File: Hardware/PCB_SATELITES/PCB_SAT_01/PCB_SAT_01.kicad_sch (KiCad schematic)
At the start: 41 parts, among them IC1 OPT3001DNPRQ1, IC2 OPT3001DNPRQ1, IC3 OPT3001DNPRQ1, IC4 OPT3001DNPRQ1, J1 MTJ-88ARX1-FSM-LG

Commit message: Actualizacion PCB SATELITE 1
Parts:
- C1, C2, C3, C4: footprint (none) -> Capacitor_SMD:C_0805_2012Metric
- J1: footprint MTJ88ARX1FSMLG -> MTJ-88ARX1-FSM-LG:MTJ88ARX1FSMLG
- R1, R10, R11, R12, R2, R3, R4, R5, R6, R7, R8, R9: footprint (none) -> Resistor_SMD:R_0805_2012Metric
- TP1_1, TP1_2, TP1_3, TP1_4, TP1_5, TP2_1, TP2_2, TP2_3, TP2_4, TP2_5, TP3_1, TP3_2, TP3_3, TP3_4, TP3_5, TP4_1, TP4_2, TP4_3, TP4_4, TP4_5: footprint (none) -> TestPoint:TestPoint_Pad_D1.0mm
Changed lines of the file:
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@@
 			)
 		)
-		(property "Footprint" ""
+		(property "Footprint" "TestPoint:TestPoint_Pad_D1.0mm"
 			(at 143.51 41.91 0)
 			(effects
@@
 			)
 		)
-		(property "Footprint" ""
+		(property "Footprint" "TestPoint:TestPoint_Pad_D1.0mm"
 			(at 92.71 49.53 0)
 			(effects
@@
 			)
 		)
-		(property "Footprint" ""
+		(property "Footprint" "TestPoint:TestPoint_Pad_D1.0mm"
 			(at 100.33 109.22 0)
 			(effects
@@
 			)
 		)
-		(property "Footprint" ""
+		(property "Footprint" "Capacitor_SMD:C_0805_2012Metric"
 			(at 155.9052 97.79 0)
 			(effects
@@
 			)
 		)
-		(property "Footprint" ""
+		(property "Footprint" "TestPoint:TestPoint_Pad_D1.0mm"
 			(at 186.69 52.07 0)
 			(effects
@@
 			)
 		)
-		(property "Footprint" ""
+		(property "Footprint" "TestPoint:TestPoint_Pad_D1.0mm"
 			(at 40.64 104.14 0)
 			(effects
@@
 			)
 		)
-		(property "Footprint" ""
+		(property "Footprint" "Capacitor_SMD:C_0805_2012Metric"
 			(at 50.4952 34.29 0)
 			(effects
@@
 			)
 		)
-		(property "Footprint" ""
+		(property "Footprint" "TestPoint:TestPoint_Pad_D1.0mm"
 			(at 195.58 49.53 0)
 			(effects
@@
 			)
 		)
-		(property "Footprint" ""
+		(property "Footprint" "Resistor_SMD:R_0805_2012Metric"
 			(at 195.072 36.83 90)
 			(effects
@@
 			)
 		)
-		(property "Footprint" ""
+		(property "Footprint" "Resistor_SMD:R_0805_2012Metric"
 			(at 99.822 36.83 90)
 			(effects
@@
 			)
 		)
-		(property "Footprint" ""
+		(property "Footprint" "TestPoint:TestPoint_Pad_D1.0mm"
 			(at 83.82 114.3 0)
 			(effects
@@
 			)
 		)
-		(property "Footprint" ""
+		(property "Footprint" "Resistor_SMD:R_0805_2012Metric"
 			(at 187.452 36.83 90)
 			(effects
@@
 			)
 		)
-		(property "Footprint" ""
+		(property "Footprint" "Capacitor_SMD:C_0805_2012Metric"
 			(at 153.3652 34.29 0)
 			(effects
@@
 			)
 		)
-		(property "Footprint" ""
+		(property "Footprint" "TestPoint:TestPoint_Pad_D1.0mm"
 			(at 189.23 115.57 0)
 			(effects
@@
 			)
 		)
-		(property "Footprint" ""
+		(property "Footprint" "Resistor_SMD:R_0805_2012Metric"
 			(at 92.202 99.06 90)
 			(effects
@@
 			)
 		)
-		(property "Footprint" ""
+		(property "Footprint" "Resistor_SMD:R_0805_2012Metric"
 			(at 189.992 100.33 90)
 			(effects
@@
 			)
 		)
-		(property "Footprint" ""
+		(property "Footprint" "Resistor_SMD:R_0805_2012Metric"
 			(at 92.202 36.83 90)
 			(effects
@@
 			)
 		)
-		(property "Footprint" ""
+		(property "Footprint" "TestPoint:TestPoint_Pad_D1.0mm"
 			(at 203.2 46.99 0)
 			(effects
@@
 			)
 		)
-		(property "Footprint" ""
+		(property "Footprint" "TestPoint:TestPoint_Pad_D1.0mm"
 			(at 100.33 46.99 0)
 			(effects
@@
 			)
 		)
-		(property "Footprint" ""
+		(property "Footprint" "TestPoint:TestPoint_Pad_D1.0mm"
 			(at 92.71 111.76 0)
 			(effects
@@
 			)
 		)
-		(property "Footprint" ""
+		(property "Footprint" "TestPoint:TestPoint_Pad_D1.0mm"
 			(at 40.64 109.22 0)
 			(effects
@@
 			)
 		)
-		(property "Footprint" ""
+		(property "Footprint" "TestPoint:TestPoint_Pad_D1.0mm"
 			(at 143.51 46.99 0)
 			(effects
@@
 			)
 		)
-		(property "Footprint" ""
+		(property "Footprint" "Capacitor_SMD:C_0805_2012Metric"
 			(at 50.4952 96.52 0)
 			(effects
@@
 			)
 		)
-		(property "Footprint" ""
+		(property "Footprint" "TestPoint:TestPoint_Pad_D1.0mm"
 			(at 83.8347 52.07 0)
 			(effects
@@
 			)
 		)
-		(property "Footprint" ""
+		(property "Footprint" "Resistor_SMD:R_0805_2012Metric"
 			(at 205.232 100.33 90)
 			(effects
@@
 			)
 		)
-		(property "Footprint" "MTJ88ARX1FSMLG"
+		(property "Footprint" "MTJ-88ARX1-FSM-LG:MTJ88ARX1FSMLG"
 			(at 274.32 191.44 0)
 			(effects
@@
 			)
 		)
-		(property "Footprint" ""
+		(property "Footprint" "TestPoint:TestPoint_Pad_D1.0mm"
 			(at 146.05 105.41 0)
 			(effects
@@
 			)
 		)
-		(property "Footprint" ""
+		(property "Footprint" "TestPoint:TestPoint_Pad_D1.0mm"
 			(at 198.12 113.03 0)
 			(effects
@@
 			)
 		)
-		(property "Footprint" ""
+		(property "Footprint" "Resistor_SMD:R_0805_2012Metric"
 			(at 84.582 99.06 90)
 			(effects
@@
 			)
 		)
-		(property "Footprint" ""
+		(property "Footprint" "TestPoint:TestPoint_Pad_D1.0mm"
 			(at 40.64 41.91 0)
 			(effects
@@
 			)
 		)
-		(property "Footprint" ""
+		(property "Footprint" "Resistor_SMD:R_0805_2012Metric"
 			(at 197.612 100.33 90)
 			(effects
@@
 			)
 		)
-		(property "Footprint" ""
+		(property "Footprint" "Resistor_SMD:R_0805_2012Metric"
 			(at 84.582 36.83 90)
 			(effects
@@
 			)
 		)
-		(property "Footprint" ""
+		(property "Footprint" "TestPoint:TestPoint_Pad_D1.0mm"
 			(at 204.47 110.49 0)
 			(effects
@@
 			)
 		)
-		(property "Footprint" ""
+		(property "Footprint" "Resistor_SMD:R_0805_2012Metric"
 			(at 202.692 36.83 90)
 			(effects
@@
 			)
 		)
-		(property "Footprint" ""
+		(property "Footprint" "TestPoint:TestPoint_Pad_D1.0mm"
 			(at 146.05 110.49 0)
 			(effects
@@
 			)
 		)
-		(property "Footprint" ""
+		(property "Footprint" "TestPoint:TestPoint_Pad_D1.0mm"
 			(at 40.64 46.99 0)
 			(effects
@@
 			)
 		)
-		(property "Footprint" ""
+		(property "Footprint" "Resistor_SMD:R_0805_2012Metric"
 			(at 99.822 99.06 90)
 			(effects

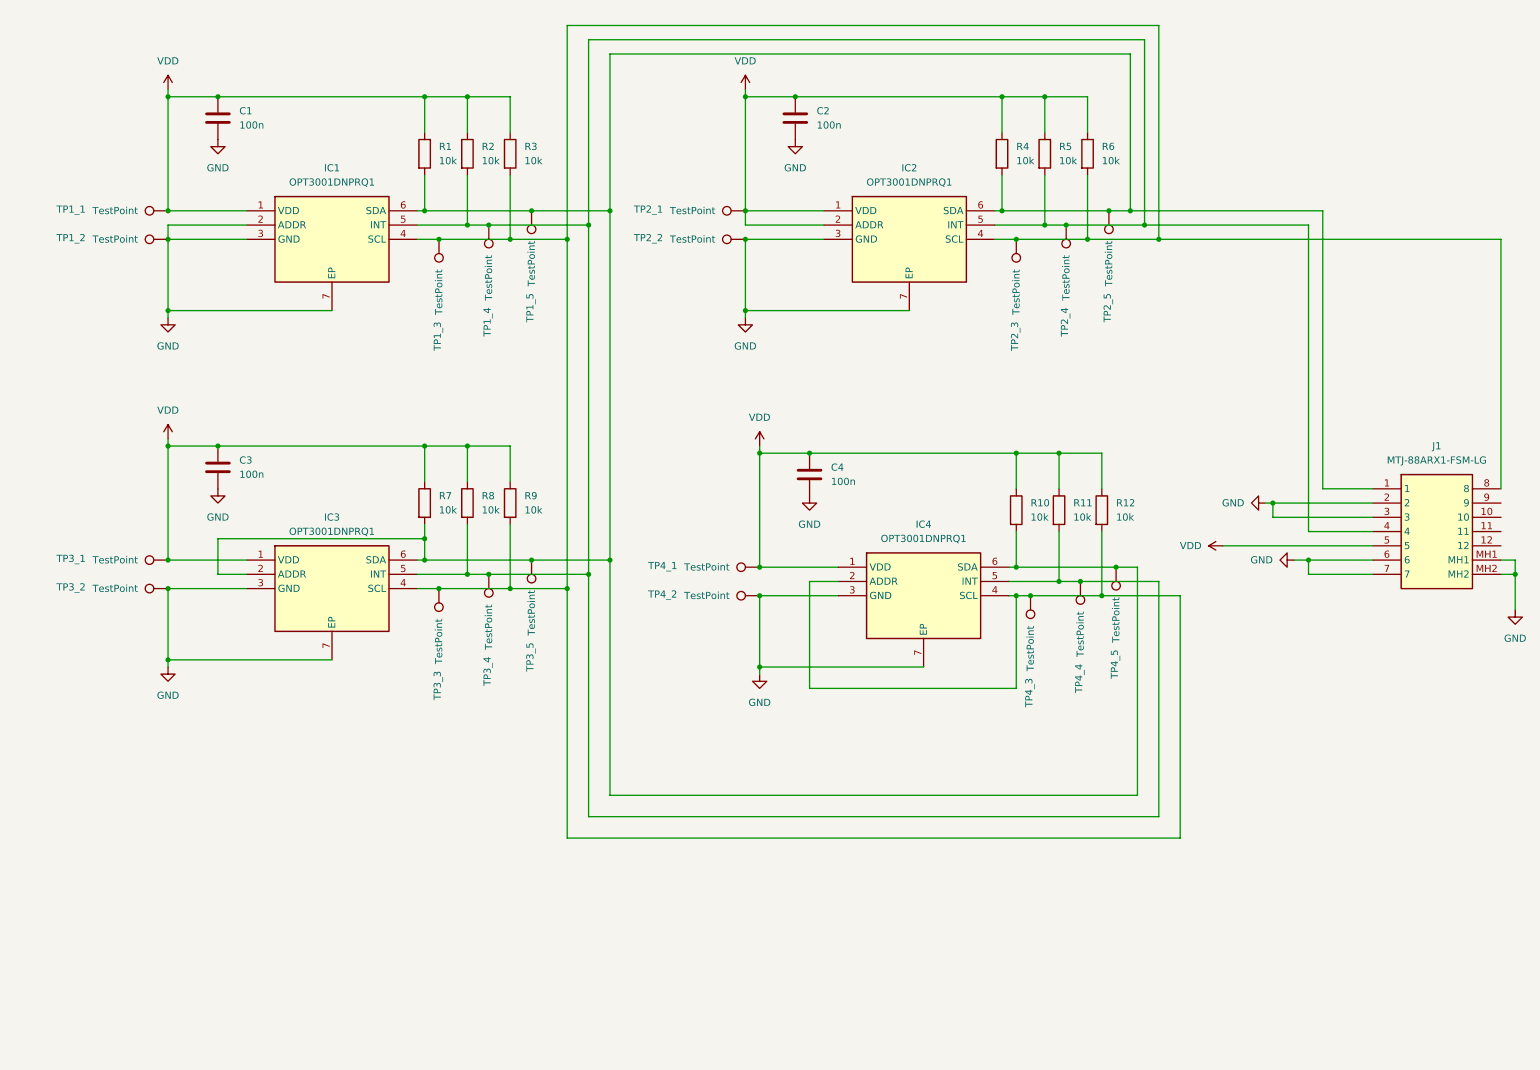
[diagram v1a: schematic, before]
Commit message: Actualizacion PCB SATELITE 1
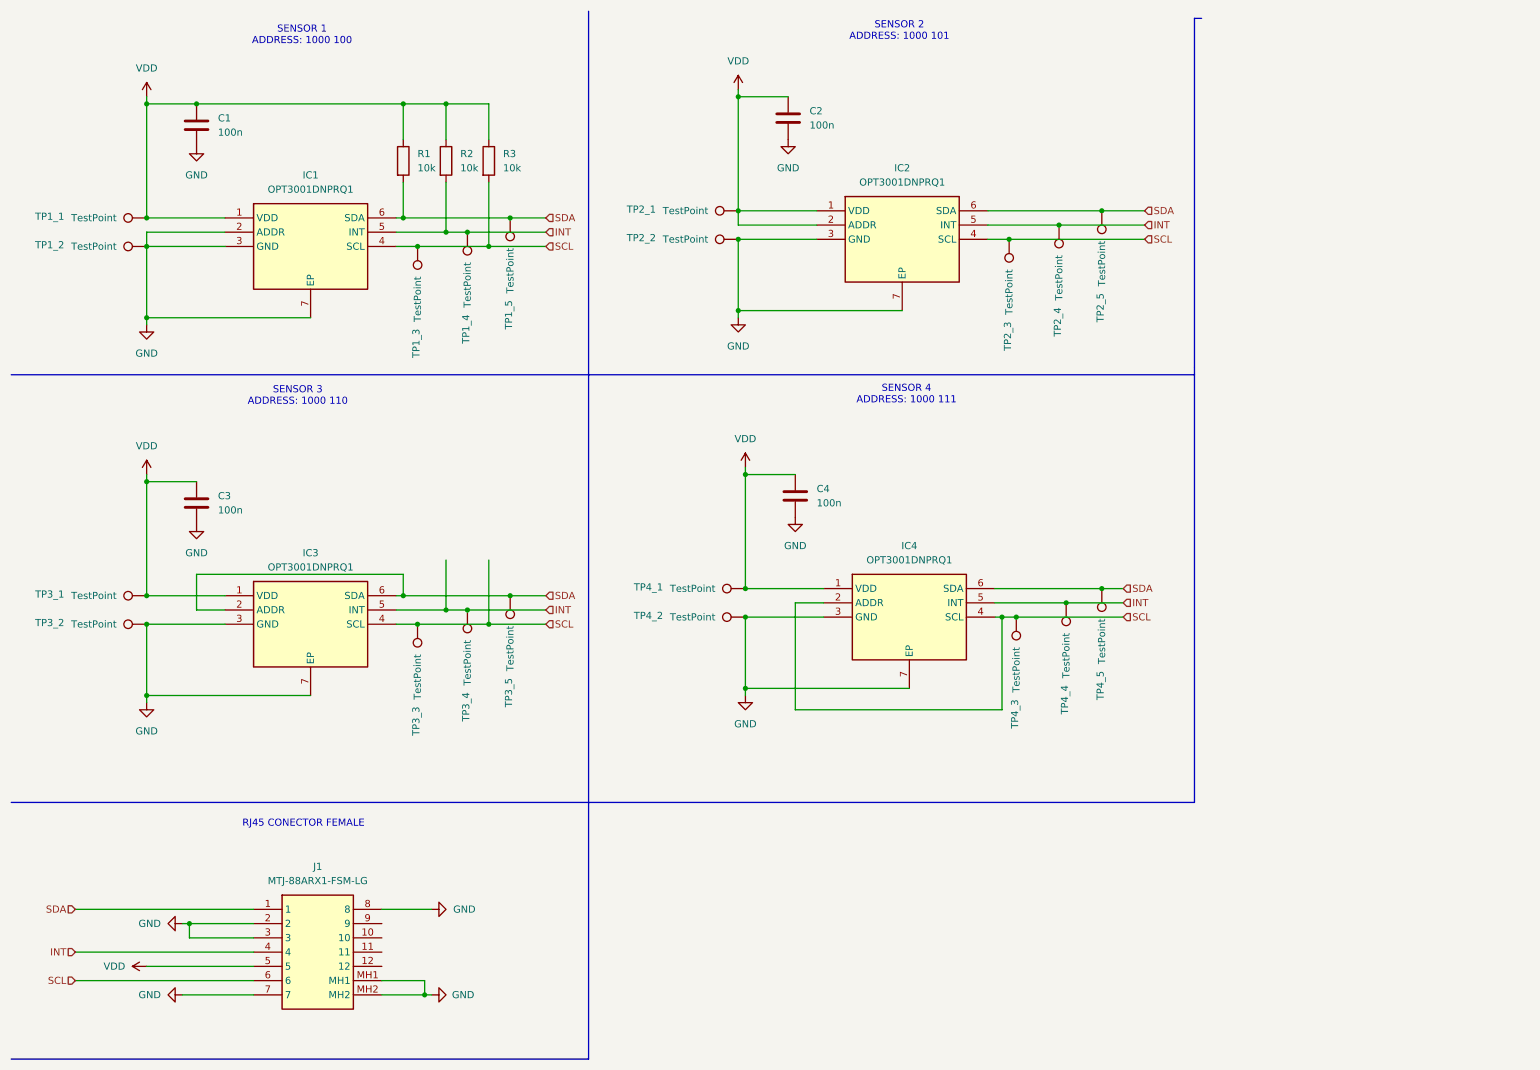
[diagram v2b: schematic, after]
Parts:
- removed R10, R11, R12, R4, R5, R6, R7, R8, R9: 10k, Resistor_SMD:R_0805_2012Metric, symbol Device:R
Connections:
- net GND: now also J1.8; no longer J1.6
- net SCL: now reaches IC1.4 (SCL), IC2.4 (SCL), IC3.4 (SCL), IC4.2 (ADDR), IC4.4 (SCL), R3.2, TP1_3.1, TP2_3.1, TP3_3.1, TP4_3.1
- net SCL: now also J1.6; no longer J1.8
- net INT: now reaches IC1.5 (INT), IC2.5 (INT), IC3.5 (INT), IC4.5 (INT), J1.4, R2.2, TP1_4.1, TP2_4.1, TP3_4.1, TP4_4.1
- net SDA: now reaches IC1.6 (SDA), IC2.6 (SDA), IC3.2 (ADDR), IC3.6 (SDA), IC4.6 (SDA), J1.1, R1.2, TP1_5.1, TP2_5.1, TP3_5.1, TP4_5.1
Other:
- note added: "RJ45 CONECTOR FEMALE"
- note added: "SENSOR 1 ADDRESS: 1000 100"
- note added: "SENSOR 2 ADDRESS: 1000 101"
- note added: "SENSOR 3 ADDRESS: 1000 110"
- note added: "SENSOR 4 ADDRESS: 1000 111"
- moved on the sheet: C1, C2, C3, C4, IC1, IC2, IC3, IC4, J1, R1, R2, R3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
